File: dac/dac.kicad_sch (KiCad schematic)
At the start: 41 parts, among them J1 Conn_01x14, U1 74LVC3G17, U2 74LVC3G17, U3 74LVC3G17

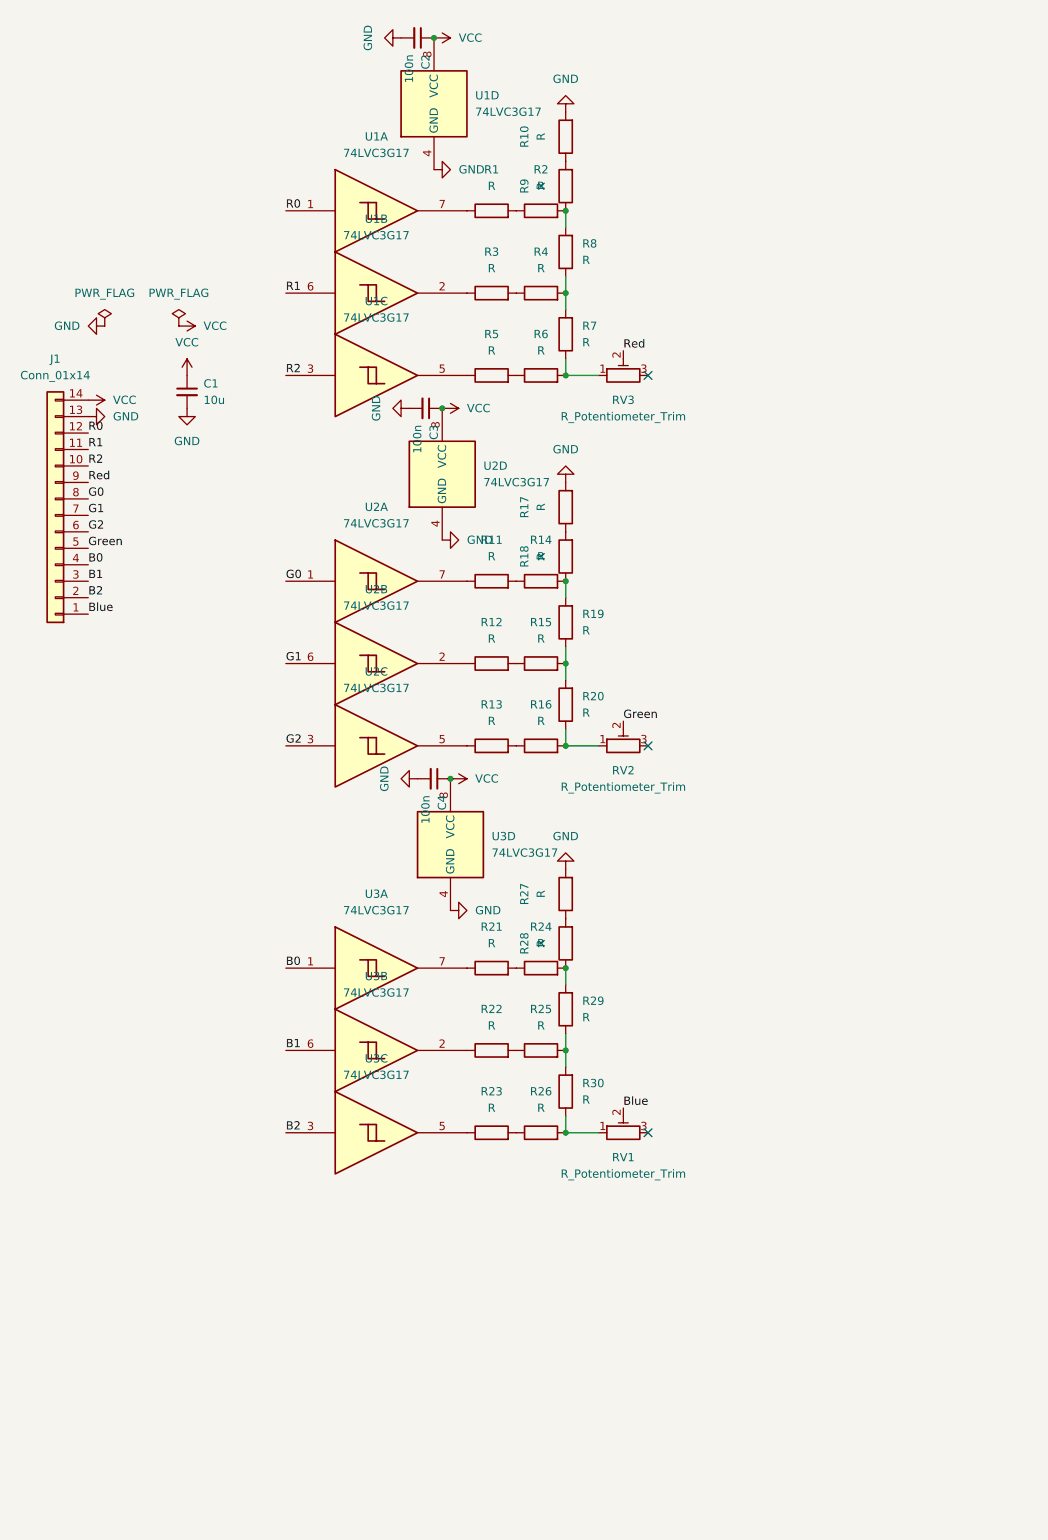
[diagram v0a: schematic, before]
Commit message: current boards
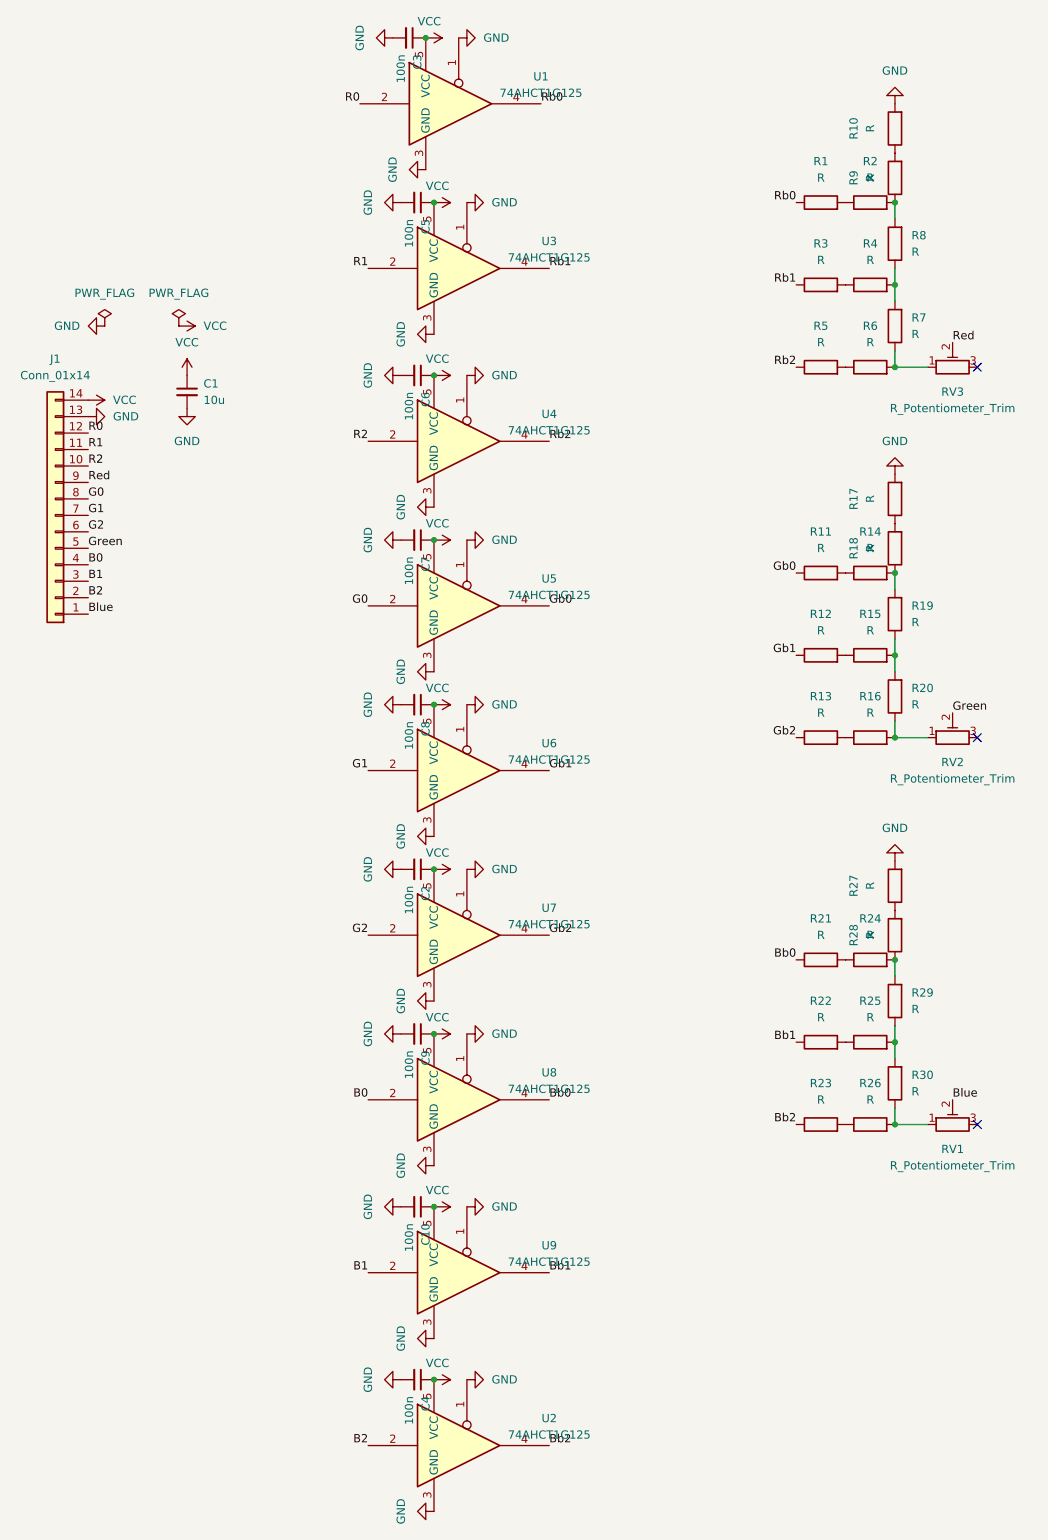
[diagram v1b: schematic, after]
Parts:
- removed U1, U2, U3: 74LVC3G17, Package_SO:VSSOP-8_3.0x3.0mm_P0.65mm, symbol 74xGxx:74LVC3G17
- added C10, C5, C6, C7, C8, C9: 100n, Capacitor_SMD:C_0805_2012Metric_Pad1.18x1.45mm_HandSolder, symbol Device:C_Small
- added U1, U2, U3, U4, U5, U6, U7, U8, U9: 74AHCT1G125, Package_TO_SOT_SMD:SOT-353_SC-70-5_Handsoldering, symbol 74xGxx:74AHCT1G125
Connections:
- net B0: now also U8.2
- net B1: now also U9.2
- net B2: now also U2.2
- net G0: now also U5.2
- net G1: now also U6.2
- net G2: now also U7.2
- net GND: now also C10.2, C5.2, C6.2, C7.2, C8.2, C9.2, U1.1, U1.3 (GND), U2.1, U2.3 (GND), U3.1, U3.3 (GND), U4.1, U4.3 (GND), U5.1, U5.3 (GND), U6.1, U6.3 (GND), U7.1, U7.3 (GND), U8.1, U8.3 (GND), U9.1, U9.3 (GND)
- net R0: now also U1.2
- net R1: now also U3.2
- net R2: now also U4.2
- net VCC: now also C10.1, C5.1, C6.1, C7.1, C8.1, C9.1, U1.5 (VCC), U2.5 (VCC), U3.5 (VCC), U4.5 (VCC), U5.5 (VCC), U6.5 (VCC), U7.5 (VCC), U8.5 (VCC), U9.5 (VCC)
- net Bb0: now reaches R21.1
- net Bb0: now also U8.4
- net Gb2: now reaches R13.1
- net Gb2: now also U7.4
- net Rb2: now reaches R5.1
- net Rb2: now also U4.4
- net Rb0: now reaches R1.1
- net Rb0: now also U1.4
- net Bb1: now reaches R22.1
- net Bb1: now also U9.4
- net Bb2: now reaches R23.1
- net Bb2: now also U2.4
- net Gb0: now reaches R11.1
- net Gb0: now also U5.4
- net Rb1: now reaches R3.1
- net Rb1: now also U3.4
- net Gb1: now reaches R12.1
- net Gb1: now also U6.4
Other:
- moved on the sheet: C4, R1, R10, R11, R12, R13, R14, R15, R16, R17, R18, R19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
